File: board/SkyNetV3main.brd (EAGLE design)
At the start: 160 x 100 mm, 67 parts, among them IC1 HC_05, IC2 RF4463PRO, IC3 LPC1768, IC4 BCX17, IC5 TPS63001, IC6 MCP73871-2CCI/ML, Q1 32.768KHz, Q2 12MHz, Q3 IRLM6402, Q4 BSS138, X1 BAT

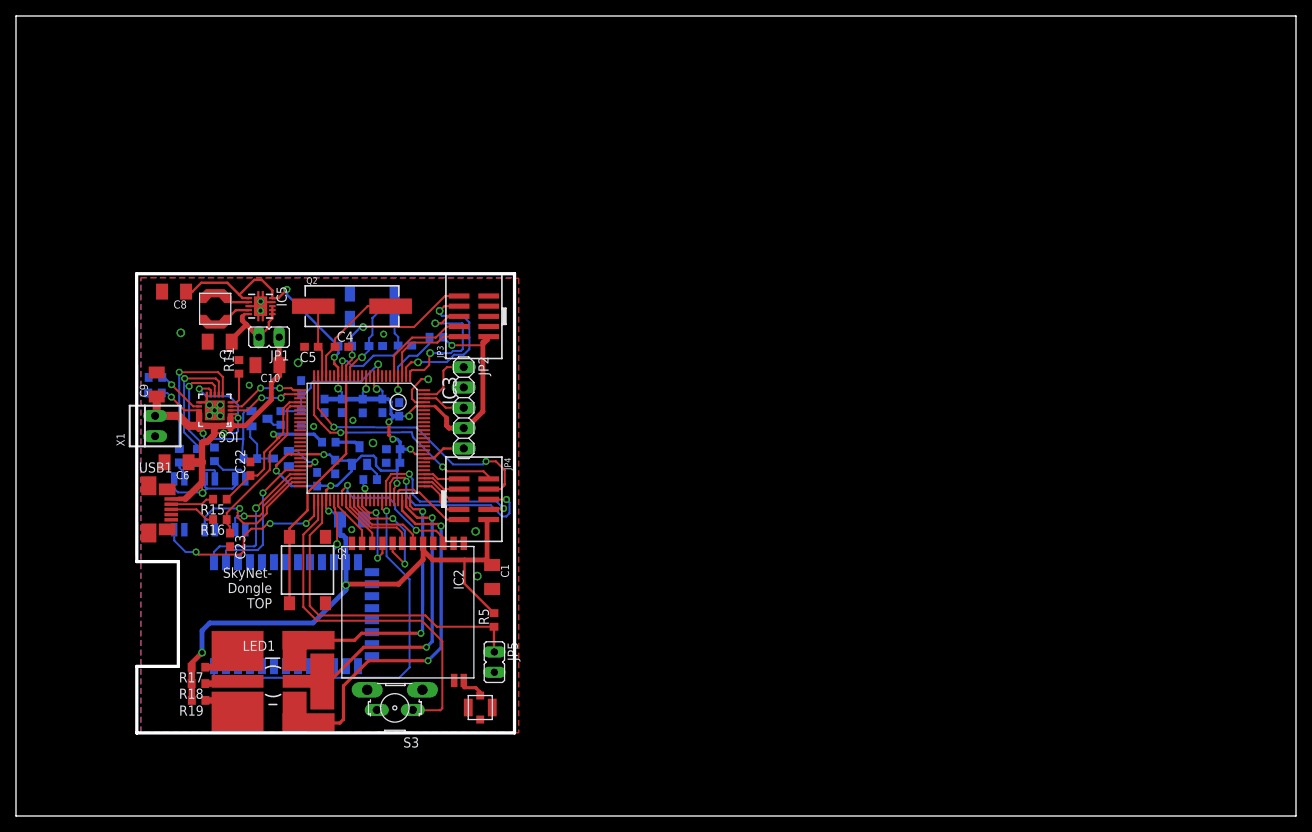
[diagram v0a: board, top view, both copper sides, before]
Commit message: new layout
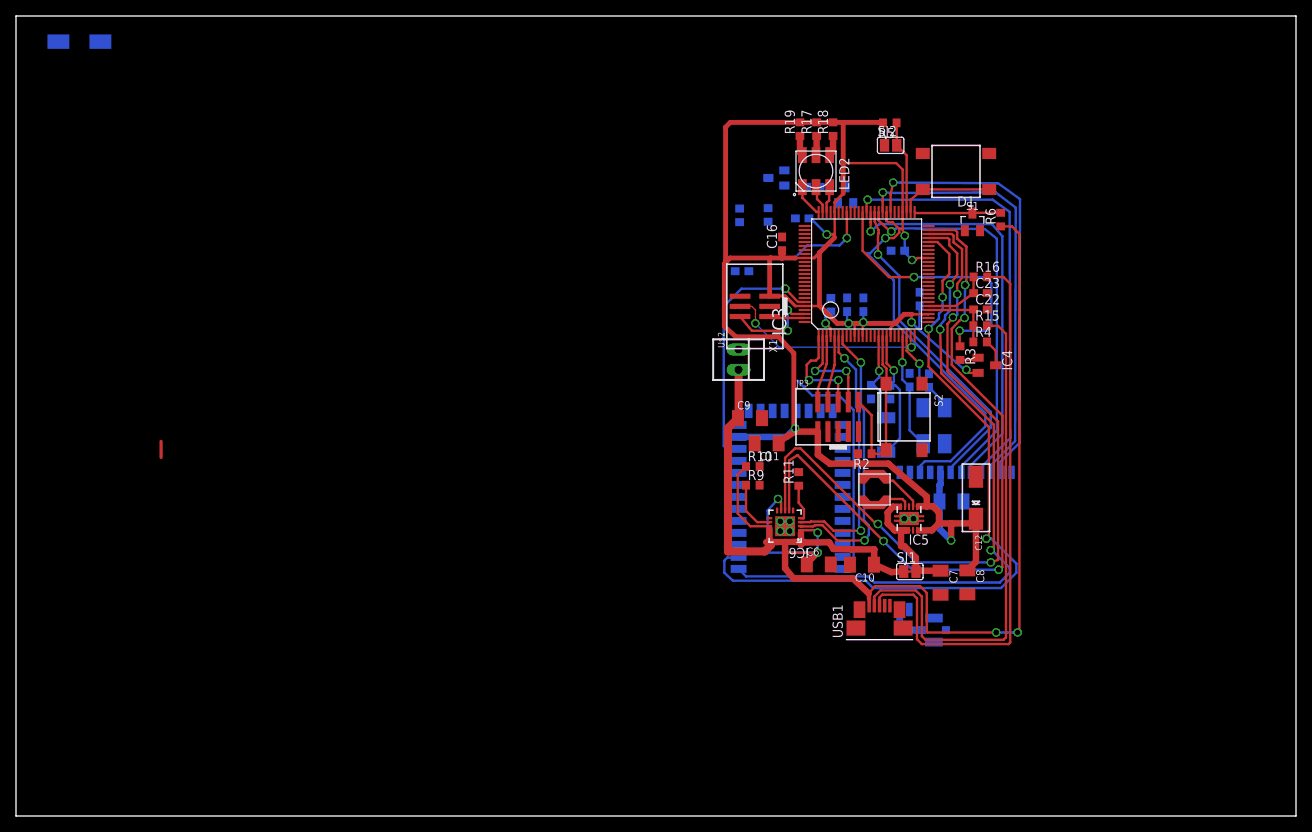
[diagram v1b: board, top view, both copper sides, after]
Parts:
- removed C14: 100n, rcl:C0603
- removed JP1: MEASURE, jumper:JP1
- removed JP2: DEBUG, pinhead:1X05
- removed JP4: PERIPH, microbuilder:2X05_1.27MM_SMT
- removed JP5: PROG, jumper:JP1
- removed LED1: STATUS, skynet_other:PLCC-6
- removed OK1, OK2, OK3: PC3H7, skynet_other:PC3H7
- removed R7, R8: 91, rcl:R0603
- removed S3: INPUT, skynet_other:PTS645-VERT
- added D1: 3v3, diode:SOT23
- added LED2: RGBLED5050, adafruit:RGBLED5050
- added S1: INPUT, switch-ck:PTS645-SMD
- added SJ1: (no value), jumper:SJ
- added SJ2: PROG, jumper:SJ
- added U$2: (no value), skynet_other:PIN-HEAD-1X3-SMD
- C12, C13: value 100n -> 100u; device rcl:C0603 -> microbuilder:EIA6032-28/C-W
- C4, C5: value 33p -> 18p
- Q1: device crystal-2:MM20SS -> skynet_other:XTAL_49_18
- Q2: device microbuilder:HC49UP -> skynet_other:XTAL_50_32
- R6: value 91 -> 10k
- moved R6 106.8 mm to (123.1, 74.5), flipped to the top, turned to 90 degrees
- moved C8 105.6 mm to (118.9, 29.2), turned to 270 degrees
- moved R18 105.3 mm to (102.1, 85.9), turned to 90 degrees
- moved R19 103.7 mm to (98.0, 85.9), turned to 90 degrees
- moved R17 102.4 mm to (100.1, 85.9), turned to 90 degrees
- moved R16 99.8 mm to (120.5, 67.4), turned to 0 degrees
- moved C23 98.7 mm to (120.5, 65.4), turned to 0 degrees
- moved R15 97.5 mm to (120.5, 61.3), turned to 0 degrees
- moved C7 95.0 mm to (115.6, 29.2), turned to 270 degrees
- moved C22 93.4 mm to (120.5, 63.3), turned to 0 degrees
- moved USB1 92.5 mm to (107.9, 23.5), turned to 90 degrees
- moved L1 85.4 mm to (105.4, 38.6)
- moved IC5 85.3 mm to (111.6, 37.2), turned to 180 degrees
- moved R4 82.4 mm to (120.5, 59.3), flipped to the top, turned to 0 degrees
- moved C6 81.3 mm to (100.4, 31.4), turned to 0 degrees
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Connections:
- net BT_AT renamed BT-AT
- net BT_RX renamed BT-RX
- net BT_TX renamed BT-TX
- net RTCX2 renamed N$2
- net SDI renamed RF-SDI
- net SPI0-NIRQ renamed RF-NIRQ
- net SPI0-NSEL renamed RF-NSEL
- net SPI0-SCLK renamed RF-SCLK
- net SPI0-SDN renamed RF-SDN
- net SPI0-SDO renamed RF-SDO
- removed net BT-RST: IC1.11, IC3.56
- removed net CHGSEL_H: IC3.27, IC6.3
- removed net CHGSEL_L: IC3.26, IC6.4
- removed net CHG_S1: IC3.48, OK3.4
- removed net CHG_S2: IC3.49, OK2.4
- removed net EXT_GPIO0: IC3.70, JP4.6
- removed net EXT_GPIO1: IC3.69, JP4.8
- removed net EXT_PWR: IC3.51, OK1.4
- removed net LED_B: IC3.73, LED1.6, LED1.6@1
- removed net LED_G: IC3.74, LED1.5, LED1.5@1
- removed net LED_R: IC3.75, LED1.4, LED1.4@1
- removed net PG: IC6.6, R6.1
- removed net PG-OK: OK1.2, R6.2
- removed net SCL_EXT: IC3.24, JP4.4
- removed net SDA_EXT: IC3.25, JP4.2
- removed net SPI2_MISO: IC3.77, JP4.5
- removed net SPI2_MOSI: IC3.76, JP4.7
- removed net SPI2_SCK: IC3.78, JP4.3
- removed net SPI2_SEL: IC3.79, JP4.1
- removed net STAT1: IC6.8, R8.1
- removed net STAT1-OK: OK3.2, R8.2
- removed net STAT2: IC6.7, R7.1
- removed net STAT2-OK: OK2.2, R7.2
- new net BT-RESET: IC1.11, IC3.95
- new net CHG-S1: IC3.48, IC6.8
- new net CHG-S2: IC3.49, IC6.7
- new net CHGSEL-H: IC3.7, IC6.3
- new net CHGSEL-L: IC3.6, IC6.4
- new net EXT-PWR: D1.3, IC3.51, R6.2
- new net LED-B: IC3.75, LED2.4
- new net LED-G: IC3.73, LED2.6
- new net LED-R: IC3.74, LED2.5
- new net SCL-EXT: IC3.24, U$2.4
- new net SDA-EXT: IC3.25, U$2.3
- net +3V3: now also C12.+, C13.+, U$2.5; no longer C12.1, C13.1, C14.1, JP2.4, JP4.10
- net +5V: now also R6.1; no longer OK1.1, OK2.1, OK3.1
- net GND: now also C12.-, C13.-, D1.1, S1.3, S1.4, SJ2.1, U$2.6; no longer C12.2, C13.2, C14.2, JP2.5, JP4.9, JP5.2, OK1.3, OK2.3, OK3.3, S3.2
- net INPUT: now also S1.1, S1.2; no longer S3.1
- net LED-B-R: now also LED2.3; no longer LED1.3
- net LED-G-R: now also LED2.1; no longer LED1.2
- net LED-R-R: now also LED2.2; no longer LED1.1
- net OUT2: now also SJ1.1; no longer JP1.1
- net PROG: now also SJ2.2; no longer JP5.1
- net RTCX1: now also Q1.2; no longer Q1.4
- net RX: now also U$2.1; no longer JP2.1
- net TX: now also U$2.2; no longer JP2.3
- net VCC: now also SJ1.2; no longer JP1.2
- net XTAL1: now also Q2.3; no longer Q2.2
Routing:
- net CHG-S2: track 0.00 -> 88.7 mm, vias 0 -> 4
- net CHG-S1: track 0.00 -> 87.3 mm, vias 0 -> 4
- net +5V: track 44.3 -> 120.7 mm, vias 4 -> 5
- net BT-RX: track 18.7 -> 90.8 mm, vias 1 -> 3
- net BT-TX: track 18.7 -> 84.7 mm, vias 1 -> 3
- net USB-D-_IN: track 5.77 -> 71.2 mm
- net USB-D+_IN: track 5.50 -> 64.2 mm
- net RF-SDN: track 6.82 -> 55.4 mm, vias 0 -> 1
- net LED_B: track 47.5 -> 0.00 mm, vias 2 -> 0
- net RF-NIRQ: track 6.98 -> 54.1 mm, vias 0 -> 1
- net RF-NSEL: track 10.7 -> 53.9 mm, vias 2 -> 1
- net LED_G: track 38.7 -> 0.00 mm, vias 2 -> 0
- net RF-SDI: track 10.2 -> 48.0 mm, vias 0 -> 1
- net CHGSEL-H: track 0.00 -> 35.9 mm, vias 0 -> 2
- net RF-SCLK: track 15.2 -> 51.1 mm, vias 2 -> 1
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- removed copper zone on layer 1, net GND
- removed copper zone on layer 16, net GND
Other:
- outline, holes or cut-outs redrawn
- board text added: "14650"
- board text added: "2x 18650"
- board text removed: "SkyNet- Dongle TOP"
- board text removed: "SkyNet-Dongle BOTTOM"
